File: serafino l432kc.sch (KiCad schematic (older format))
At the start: 31 parts, among them J1 USB_B_Micro, J2 Conn_01x14, J3 Conn_01x14, Q1 SI3401A-TP, SW1 SW_Push, SW2 SW_Push, U1 AP2112K-3.3, U2 USBLC6-2SC6, U3 STM32L432KCUx, Y1 32.768K

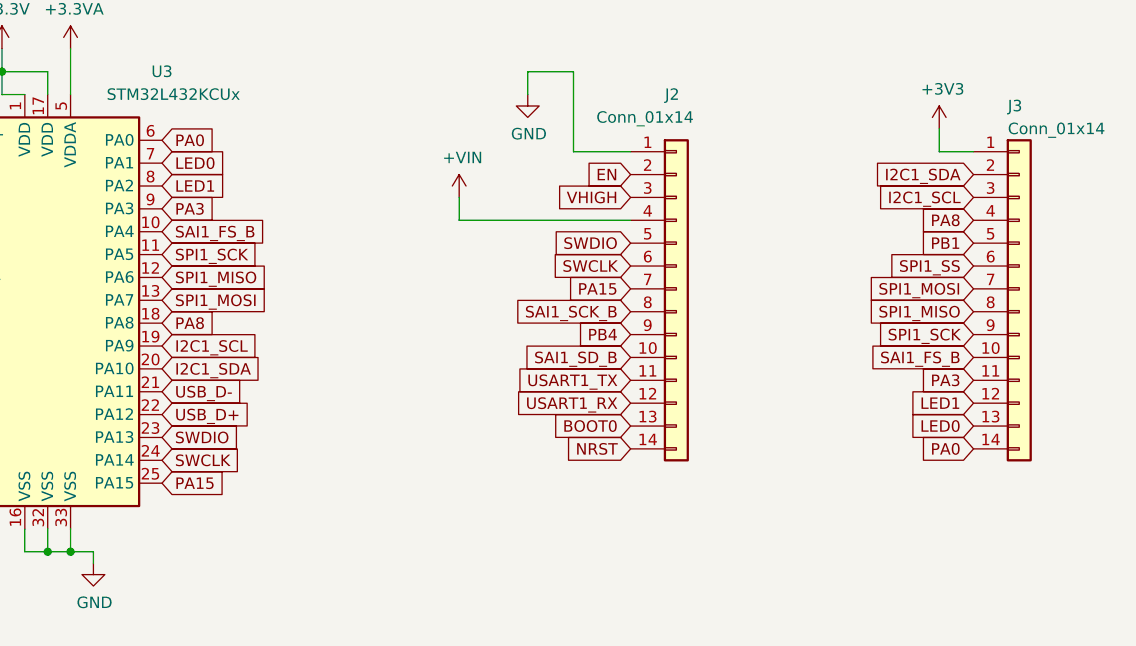
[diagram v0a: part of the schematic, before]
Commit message: Avances
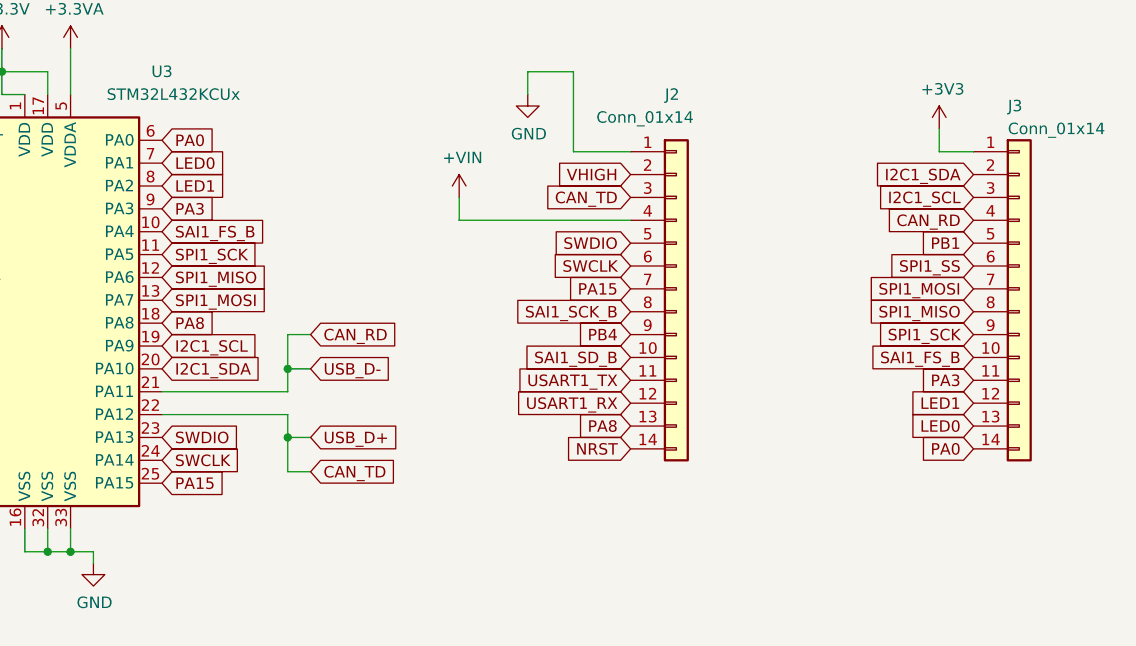
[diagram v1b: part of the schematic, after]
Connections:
- net BOOT0: no longer J2.13 (Pin_13)
- net EN: no longer J2.2 (Pin_2)
- net PA8: now also J2.13 (Pin_13); no longer J3.4 (Pin_4)
- net VHIGH: now also J2.2 (Pin_2); no longer J2.3 (Pin_3)
- net USB_D+ renamed CAN_TD
- net CAN_TD: now also J2.3 (Pin_3)
- net USB_D- renamed CAN_RD
- net CAN_RD: now also J3.4 (Pin_4)
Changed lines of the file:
@@
 Text GLabel 6700 4800 2    50   Input ~ 0
 SWCLK
-Text GLabel 6700 4600 2    50   Input ~ 0
+Text GLabel 7350 4700 2    50   Input ~ 0
 USB_D+
-Text GLabel 6700 4500 2    50   Input ~ 0
+Text GLabel 7350 4400 2    50   Input ~ 0
 USB_D-
 Text GLabel 5700 4800 0    50   Input ~ 0
@@
 	1    0    0    -1
 $EndComp
-Text GLabel 8750 3650 0    50   Input ~ 0
+Text GLabel 8750 3550 0    50   Input ~ 0
 VHIGH
 Text GLabel 8750 4750 0    50   Input ~ 0
 NRST
-Text GLabel 10250 3750 0    50   Input ~ 0
+Text GLabel 8750 4650 0    50   Input ~ 0
 PA8
 Text GLabel 8750 4050 0    50   Input ~ 0
@@
 Text GLabel 10250 3950 0    50   Input ~ 0
 SPI1_SS
-Text GLabel 8750 4250 0    50   Input ~ 0
-PB4
 Text GLabel 10250 4650 0    50   Input ~ 0
 LED0
@@
 Text GLabel 10250 4350 0    50   Input ~ 0
 SAI1_FS_B
-Text GLabel 8750 4550 0    50   Input ~ 0
-USART1_RX
-Text GLabel 8750 4450 0    50   Input ~ 0
-USART1_TX
 Text GLabel 10250 4250 0    50   Input ~ 0
 SPI1_SCK
@@
 Wire Wire Line
 	8500 3450 8750 3450
-Text GLabel 8750 4650 0    50   Input ~ 0
-BOOT0
 $Comp
 L Device:R_Small R3
@@
 Text GLabel 8750 4150 0    50   Input ~ 0
 SAI1_SCK_B
-Text GLabel 8750 3550 0    50   Input ~ 0
-EN
 Wire Wire Line
 	2250 4600 2900 4600
@@
 Text GLabel 5700 4700 0    50   Input ~ 0
 SAI1_SD_B
-Text GLabel 8750 4350 0    50   Input ~ 0
-SAI1_SD_B
-$Comp
-L power:+3.3V #PWR?
+$Comp
+L power:+3.3V #PWR0107
 U 1 1 6018DE27
 P 3850 5700
-F 0 "#PWR?" H 3850 5550 50  0001 C CNN
+F 0 "#PWR0107" H 3850 5550 50  0001 C CNN
 F 1 "+3.3V" H 3865 5873 50  0000 C CNN
 F 2 "" H 3850 5700 50  0001 C CNN
@@
 Text Notes 1500 6100 0    50   ~ 0
 * LED for Native \nDFU Mode Indicator
+Text GLabel 8750 4250 0    50   Input ~ 0
+PB4
+Text GLabel 8750 4350 0    50   Input ~ 0
+SAI1_SD_B
+Text GLabel 8750 4450 0    50   Input ~ 0
+USART1_TX
+Text GLabel 8750 4550 0    50   Input ~ 0
+USART1_RX
+Text GLabel 8750 3650 0    50   Input ~ 0
+CAN_TD
+Text GLabel 10250 3750 0    50   Input ~ 0
+CAN_RD
+Wire Wire Line
+	7350 4400 7250 4400
+Wire Wire Line
+	7250 4400 7250 4500
+Wire Wire Line
+	7250 4500 6700 4500
+Wire Wire Line
+	7350 4700 7250 4700
+Wire Wire Line
+	7250 4700 7250 4600
+Wire Wire Line
+	7250 4600 6700 4600
+Text GLabel 7350 4850 2    50   Input ~ 0
+CAN_TD
+Text GLabel 7350 4250 2    50   Input ~ 0
+CAN_RD
+Wire Wire Line
+	7350 4250 7250 4250
+Wire Wire Line
+	7250 4250 7250 4400
+Connection ~ 7250 4400
+Wire Wire Line
+	7350 4850 7250 4850
+Wire Wire Line
+	7250 4850 7250 4700
+Connection ~ 7250 4700
 $EndSCHEMATC
